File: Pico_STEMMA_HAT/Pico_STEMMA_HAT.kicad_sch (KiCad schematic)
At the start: 57 parts, among them J1 Conn_01x20_Socket, J2 Conn_01x20_Socket, J3 SDCARD_MODULE

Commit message: Update schematic formatting
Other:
- note added: "Neopixel"
- note added: "RASPBERRY PI PICO HEADER CONNECTIONS"
- note removed: "MQTT STATUS NEOPIXEL"
- note removed: "RASPBERRY PI PICO W HEADER CONNECTIONS"
- moved on the sheet: C1, C10, C2, C3, C4, C5, C6, C7, C8, C9, D1, D2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

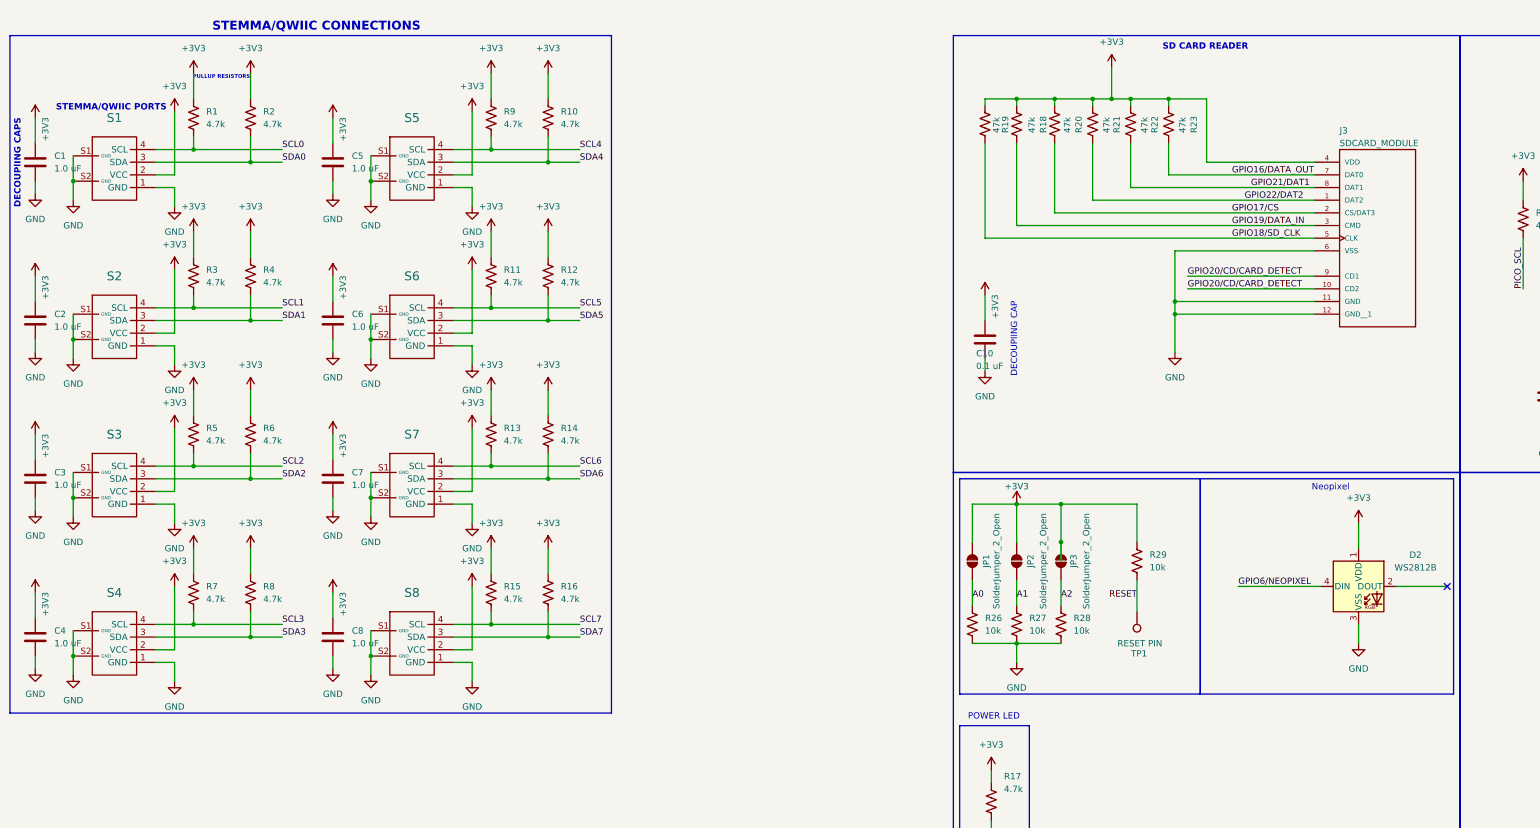
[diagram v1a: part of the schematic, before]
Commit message: Update schematic
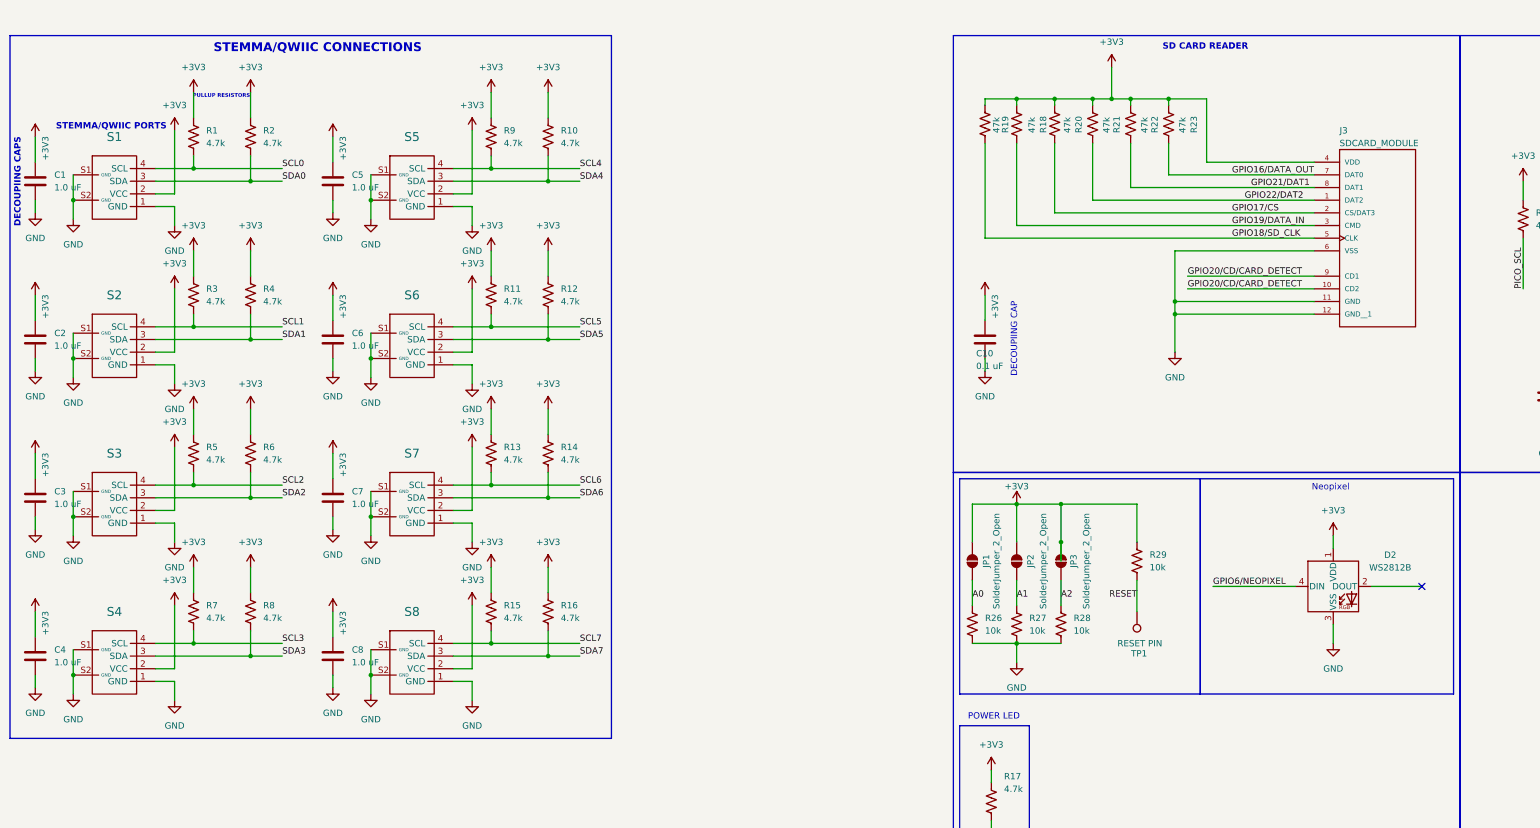
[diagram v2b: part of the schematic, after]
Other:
- moved on the sheet: C1, C2, C3, C4, C5, C6, C7, C8, R1, R10, R11, R12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
